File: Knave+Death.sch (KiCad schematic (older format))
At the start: 42 parts, among them J1 OUT0_3.5mm, J2 OUT1_3.5mm, J3 OUT2_3.5mm, J4 PWR_IN_PHNX, J5 OUT3_3.5mm, J6 E0_3.5mm, J7 E1_3.5mm, SW1 SW_SPDT, U1 LM324, U2 LM358, U3 CD4017, U4 CD4017, U5 NE555

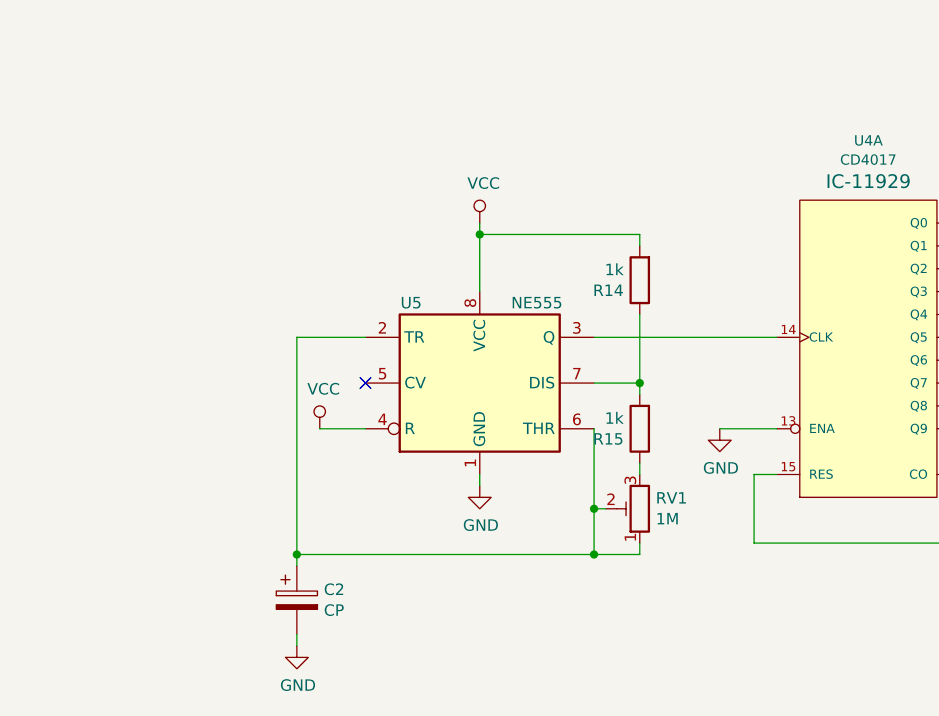
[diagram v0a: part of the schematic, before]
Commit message: commit before changing schematic
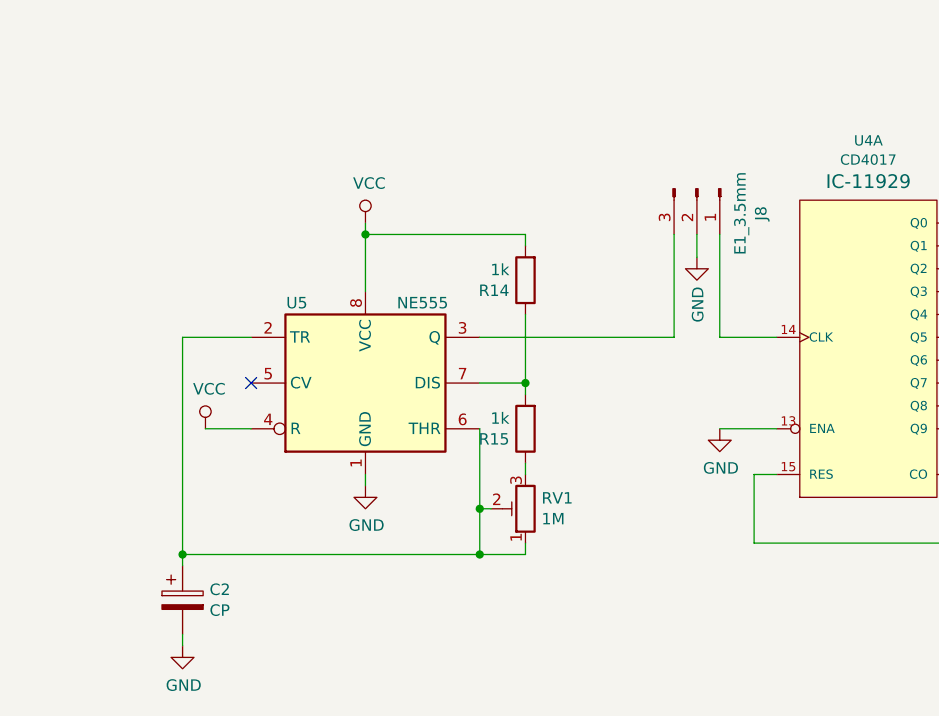
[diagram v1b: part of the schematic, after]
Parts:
- added J8: E1_3.5mm, HammerheadAudio:EuroJack_MonoSW_THT, symbol Connector:Conn_01x03_Male
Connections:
- net GND: now also J8.2 (Pin_2)
- net at U4.14 (CLK): now also J8.1 (Pin_1); no longer U5.3 (Q)
- new net: J8.3 (Pin_3), U5.3 (Q)
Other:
- moved on the sheet: C2, R14, R15, RV1, U5
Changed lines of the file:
@@
 L Timer:NE555 U5
 U 1 1 5E794E13
-P 5100 5300
-F 0 "U5" H 4800 5650 50  0000 C CNN
-F 1 "NE555" H 5350 5650 50  0000 C CNN
-F 2 "Package_DIP:DIP-8_W7.62mm_Socket" H 5100 5300 50  0001 C CNN
-F 3 "http://www.ti.com/lit/ds/symlink/ne555.pdf" H 5100 5300 50  0001 C CNN
-	1    5100 5300
-	1    0    0    -1
-$EndComp
-Wire Wire Line
-	5600 5100 6400 5100
+P 4600 5300
+F 0 "U5" H 4300 5650 50  0000 C CNN
+F 1 "NE555" H 4850 5650 50  0000 C CNN
+F 2 "Package_DIP:DIP-8_W7.62mm_Socket" H 4600 5300 50  0001 C CNN
+F 3 "http://www.ti.com/lit/ds/symlink/ne555.pdf" H 4600 5300 50  0001 C CNN
+	1    4600 5300
+	1    0    0    -1
+$EndComp
 $Comp
 L power:VCC #PWR026
 U 1 1 5E7974FB
-P 4400 5500
-F 0 "#PWR026" H 4400 5350 50  0001 C CNN
-F 1 "VCC" H 4417 5673 50  0000 C CNN
-F 2 "" H 4400 5500 50  0001 C CNN
-F 3 "" H 4400 5500 50  0001 C CNN
-	1    4400 5500
-	1    0    0    -1
-$EndComp
-NoConn ~ 4600 5300
-Wire Wire Line
-	4600 5500 4400 5500
+P 3900 5500
+F 0 "#PWR026" H 3900 5350 50  0001 C CNN
+F 1 "VCC" H 3917 5673 50  0000 C CNN
+F 2 "" H 3900 5500 50  0001 C CNN
+F 3 "" H 3900 5500 50  0001 C CNN
+	1    3900 5500
+	1    0    0    -1
+$EndComp
+NoConn ~ 4100 5300
+Wire Wire Line
+	4100 5500 3900 5500
 $Comp
 L power:GND #PWR028
 U 1 1 5E798069
-P 5100 5750
-F 0 "#PWR028" H 5100 5500 50  0001 C CNN
-F 1 "GND" H 5105 5577 50  0000 C CNN
-F 2 "" H 5100 5750 50  0001 C CNN
-F 3 "" H 5100 5750 50  0001 C CNN
-	1    5100 5750
-	1    0    0    -1
-$EndComp
-Wire Wire Line
-	5100 5750 5100 5700
+P 4600 5750
+F 0 "#PWR028" H 4600 5500 50  0001 C CNN
+F 1 "GND" H 4605 5577 50  0000 C CNN
+F 2 "" H 4600 5750 50  0001 C CNN
+F 3 "" H 4600 5750 50  0001 C CNN
+	1    4600 5750
+	1    0    0    -1
+$EndComp
+Wire Wire Line
+	4600 5750 4600 5700
 $Comp
 L Device:R R15
 U 1 1 5E7988F4
-P 5800 5500
-F 0 "R15" H 5870 5546 50  0000 L CNN
-F 1 "1k" H 5870 5455 50  0000 L CNN
-F 2 "HammerheadAudio:R_THT_P7.62" V 5730 5500 50  0001 C CNN
-F 3 "~" H 5800 5500 50  0001 C CNN
-	1    5800 5500
+P 5300 5500
+F 0 "R15" H 5370 5546 50  0000 L CNN
+F 1 "1k" H 5370 5455 50  0000 L CNN
+F 2 "HammerheadAudio:R_THT_P7.62" V 5230 5500 50  0001 C CNN
+F 3 "~" H 5300 5500 50  0001 C CNN
+	1    5300 5500
 	-1   0    0    1
 $EndComp
@@
 L Device:R R14
 U 1 1 5E799458
-P 5800 4850
-F 0 "R14" H 5870 4896 50  0000 L CNN
-F 1 "1k" H 5870 4805 50  0000 L CNN
-F 2 "HammerheadAudio:R_THT_P7.62" V 5730 4850 50  0001 C CNN
-F 3 "~" H 5800 4850 50  0001 C CNN
-	1    5800 4850
+P 5300 4850
+F 0 "R14" H 5370 4896 50  0000 L CNN
+F 1 "1k" H 5370 4805 50  0000 L CNN
+F 2 "HammerheadAudio:R_THT_P7.62" V 5230 4850 50  0001 C CNN
+F 3 "~" H 5300 4850 50  0001 C CNN
+	1    5300 4850
 	-1   0    0    1
 $EndComp
 Wire Wire Line
-	5800 5350 5800 5300
-Wire Wire Line
-	5800 5000 5800 5300
-Connection ~ 5800 5300
-Wire Wire Line
-	5100 4900 5100 4650
+	5300 5350 5300 5300
+Wire Wire Line
+	5300 5000 5300 5300
+Connection ~ 5300 5300
+Wire Wire Line
+	4600 4900 4600 4650
 $Comp
 L power:VCC #PWR022
 U 1 1 5E79A9DD
-P 5100 4600
-F 0 "#PWR022" H 5100 4450 50  0001 C CNN
-F 1 "VCC" H 5117 4773 50  0000 C CNN
-F 2 "" H 5100 4600 50  0001 C CNN
-F 3 "" H 5100 4600 50  0001 C CNN
-	1    5100 4600
-	1    0    0    -1
-$EndComp
-Wire Wire Line
-	5100 4650 5100 4600
-Connection ~ 5100 4650
+P 4600 4600
+F 0 "#PWR022" H 4600 4450 50  0001 C CNN
+F 1 "VCC" H 4617 4773 50  0000 C CNN
+F 2 "" H 4600 4600 50  0001 C CNN
+F 3 "" H 4600 4600 50  0001 C CNN
+	1    4600 4600
+	1    0    0    -1
+$EndComp
+Wire Wire Line
+	4600 4650 4600 4600
+Connection ~ 4600 4650
 $Comp
 L Device:R_POT_TRIM RV1
 U 1 1 5E79B5EB
-P 5800 5850
-F 0 "RV1" H 5730 5804 50  0000 R CNN
-F 1 "1M" H 5730 5895 50  0000 R CNN
-F 2 "Potentiometer_THT:Potentiometer_Piher_PT-6-V_Vertical" H 5800 5850 50  0001 C CNN
-F 3 "~" H 5800 5850 50  0001 C CNN
-	1    5800 5850
+P 5300 5850
+F 0 "RV1" H 5230 5804 50  0000 R CNN
+F 1 "1M" H 5230 5895 50  0000 R CNN
+F 2 "Potentiometer_THT:Potentiometer_Piher_PT-6-V_Vertical" H 5300 5850 50  0001 C CNN
+F 3 "~" H 5300 5850 50  0001 C CNN
+	1    5300 5850
 	-1   0    0    1
 $EndComp
 Wire Wire Line
-	5800 5700 5800 5650
-Wire Wire Line
-	5800 4650 5800 4700
-Wire Wire Line
-	5100 4650 5800 4650
-Wire Wire Line
-	5600 5300 5800 5300
-Wire Wire Line
-	5600 5500 5600 5850
-Wire Wire Line
-	5600 6050 4300 6050
-Wire Wire Line
-	4300 6050 4300 5100
-Wire Wire Line
-	4300 5100 4600 5100
-Wire Wire Line
-	5600 5850 5650 5850
-Connection ~ 5600 5850
-Wire Wire Line
-	5600 5850 5600 6050
-Wire Wire Line
-	5800 6000 5800 6050
-Wire Wire Line
-	5800 6050 5600 6050
-Connection ~ 5600 6050
+	5300 5700 5300 5650
+Wire Wire Line
+	5300 4650 5300 4700
+Wire Wire Line
+	4600 4650 5300 4650
+Wire Wire Line
+	5100 5300 5300 5300
+Wire Wire Line
+	5100 5500 5100 5850
+Wire Wire Line
+	5100 6050 3800 6050
+Wire Wire Line
+	3800 6050 3800 5100
+Wire Wire Line
+	3800 5100 4100 5100
+Wire Wire Line
+	5100 5850 5150 5850
+Connection ~ 5100 5850
+Wire Wire Line
+	5100 5850 5100 6050
+Wire Wire Line
+	5300 6000 5300 6050
+Wire Wire Line
+	5300 6050 5100 6050
+Connection ~ 5100 6050
 NoConn ~ 7200 5100
 NoConn ~ 7200 5200
@@
 L Device:CP C2
 U 1 1 5E7A1F2F
-P 4300 6250
-F 0 "C2" H 4418 6296 50  0000 L CNN
-F 1 "CP" H 4418 6205 50  0000 L CNN
-F 2 "Capacitor_THT:CP_Radial_D6.3mm_P2.50mm" H 4338 6100 50  0001 C CNN
-F 3 "~" H 4300 6250 50  0001 C CNN
-	1    4300 6250
+P 3800 6250
+F 0 "C2" H 3918 6296 50  0000 L CNN
+F 1 "CP" H 3918 6205 50  0000 L CNN
+F 2 "Capacitor_THT:CP_Radial_D6.3mm_P2.50mm" H 3838 6100 50  0001 C CNN
+F 3 "~" H 3800 6250 50  0001 C CNN
+	1    3800 6250
 	1    0    0    -1
 $EndComp
@@
 L power:GND #PWR029
 U 1 1 5E7A2621
-P 4300 6450
-F 0 "#PWR029" H 4300 6200 50  0001 C CNN
-F 1 "GND" H 4305 6277 50  0000 C CNN
-F 2 "" H 4300 6450 50  0001 C CNN
-F 3 "" H 4300 6450 50  0001 C CNN
-	1    4300 6450
-	1    0    0    -1
-$EndComp
-Wire Wire Line
-	4300 6100 4300 6050
-Connection ~ 4300 6050
-Wire Wire Line
-	4300 6450 4300 6400
+P 3800 6450
+F 0 "#PWR029" H 3800 6200 50  0001 C CNN
+F 1 "GND" H 3805 6277 50  0000 C CNN
+F 2 "" H 3800 6450 50  0001 C CNN
+F 3 "" H 3800 6450 50  0001 C CNN
+	1    3800 6450
+	1    0    0    -1
+$EndComp
+Wire Wire Line
+	3800 6100 3800 6050
+Connection ~ 3800 6050
+Wire Wire Line
+	3800 6450 3800 6400
 $Comp
 L SparkFun-IC-Logic:CD4017 U3
@@
 Wire Wire Line
 	8500 5050 8550 5050
+$Comp
+L Connector:Conn_01x03_Male J8
+U 1 1 5E7ABC41
+P 6050 4450
+F 0 "J8" H 6158 4731 50  0000 C CNN
+F 1 "E1_3.5mm" H 6158 4640 50  0000 C CNN
+F 2 "HammerheadAudio:EuroJack_MonoSW_THT" H 6050 4450 50  0001 C CNN
+F 3 "~" H 6050 4450 50  0001 C CNN
+	1    6050 4450
+	0    1    1    0
+$EndComp
+Wire Wire Line
+	6050 4650 6050 4750
+$Comp
+L power:GND #PWR0101
+U 1 1 5E7ABC4D
+P 6050 4750
+F 0 "#PWR0101" H 6050 4500 50  0001 C CNN
+F 1 "GND" V 6055 4622 50  0000 R CNN
+F 2 "" H 6050 4750 50  0001 C CNN
+F 3 "" H 6050 4750 50  0001 C CNN
+	1    6050 4750
+	1    0    0    -1
+$EndComp
+Wire Wire Line
+	6150 4650 6150 5100
+Wire Wire Line
+	6150 5100 6400 5100
+Wire Wire Line
+	5950 4650 5950 5100
+Wire Wire Line
+	5100 5100 5950 5100
 $EndSCHEMATC
